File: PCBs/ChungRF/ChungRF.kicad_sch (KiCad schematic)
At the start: 11 parts, among them J1 Conn_Coaxial, J2 Conn_01x09_Socket, U1 E22-900M30S

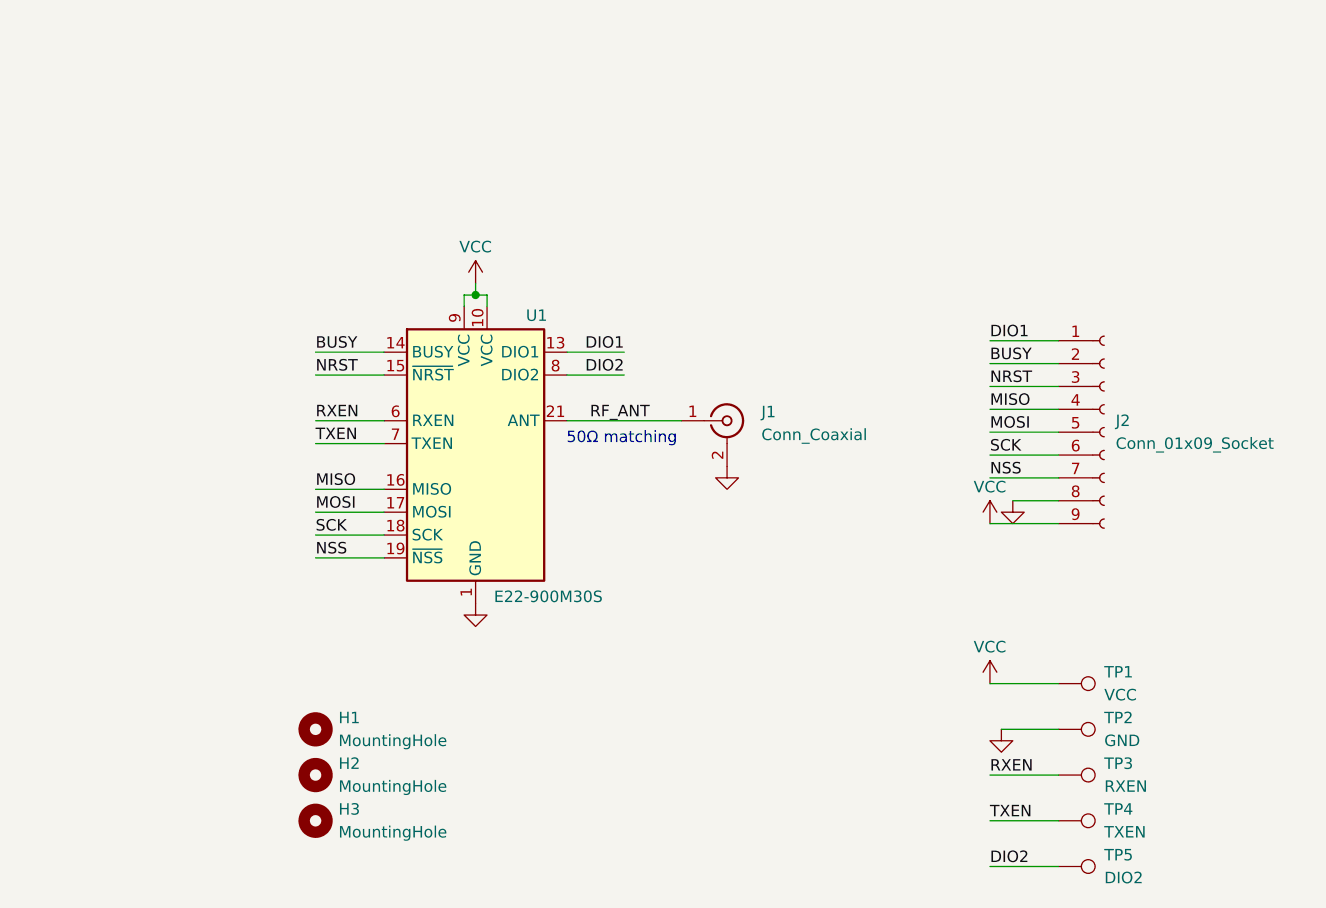
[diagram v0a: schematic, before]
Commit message: Rename to ChungRF
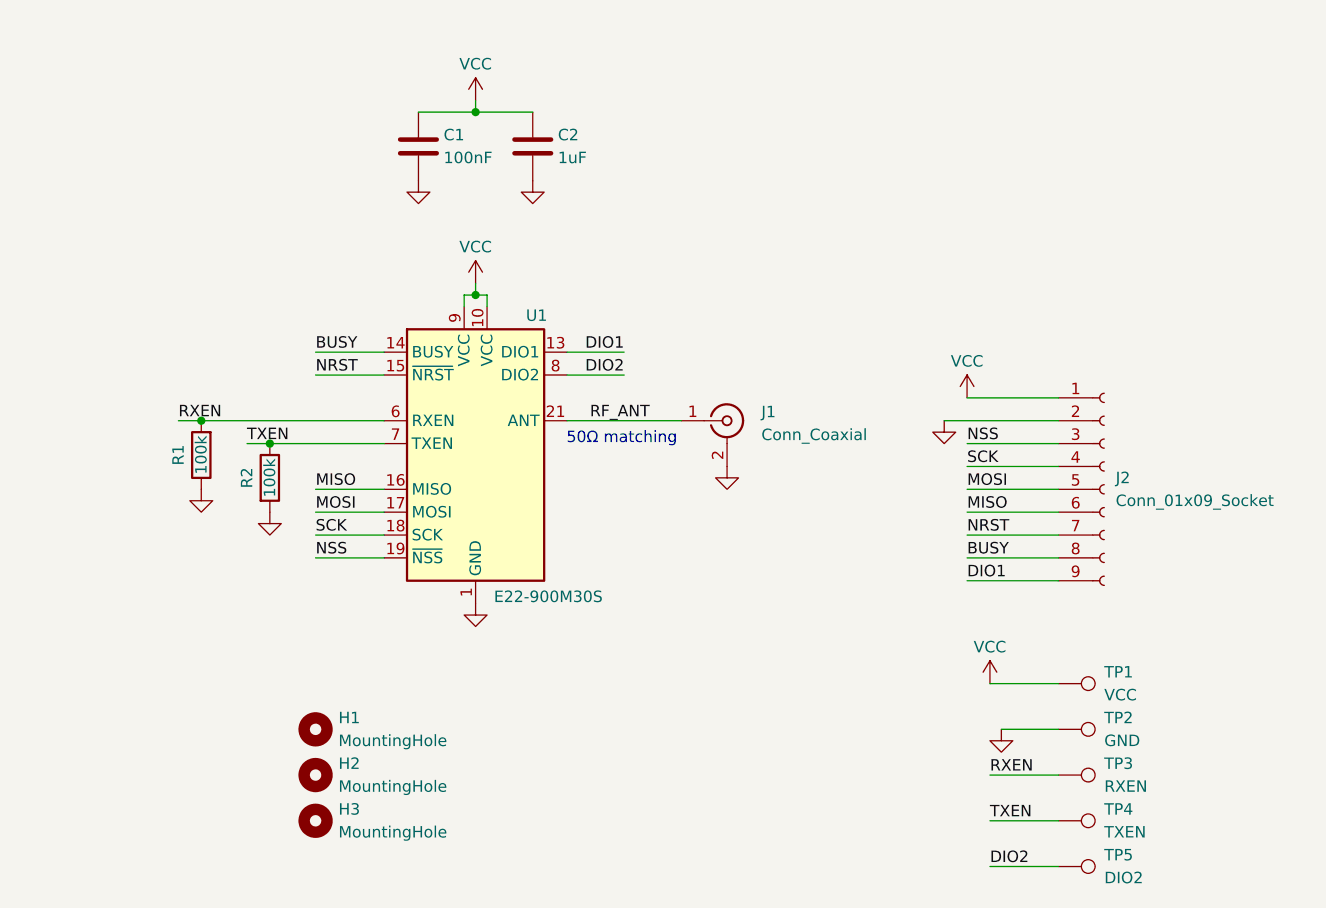
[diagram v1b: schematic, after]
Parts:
- added C1: 100nF, Capacitor_SMD:C_0603_1608Metric, symbol Device:C
- added C2: 1uF, Capacitor_SMD:C_0603_1608Metric, symbol Device:C
- added R1, R2: 100k, Capacitor_SMD:C_0603_1608Metric, symbol Device:R
- J2: footprint Connector_JST:JST_GH_BM09B-GHS-TBT_1x09-1MP_P1.25mm_Vertical -> Connector_JST:JST_SH_SM09B-SRSS-TB_1x09-1MP_P1.00mm_Horizontal
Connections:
- net BUSY: now also J2.8 (Pin_8); no longer J2.2 (Pin_2)
- net DIO1: now also J2.9 (Pin_9); no longer J2.1 (Pin_1)
- net GND: now also J2.2 (Pin_2), C1.2, C2.2, R1.1, R2.2; no longer J2.8 (Pin_8)
- net MISO: now also J2.6 (Pin_6); no longer J2.4 (Pin_4)
- net NRST: now also J2.7 (Pin_7); no longer J2.3 (Pin_3)
- net NSS: now also J2.3 (Pin_3); no longer J2.7 (Pin_7)
- net RXEN: now also R1.2
- net SCK: now also J2.4 (Pin_4); no longer J2.6 (Pin_6)
- net TXEN: now also R2.1
- net VCC: now also J2.1 (Pin_1), C1.1, C2.1; no longer J2.9 (Pin_9)
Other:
- moved on the sheet: J2

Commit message: Update ChungRF
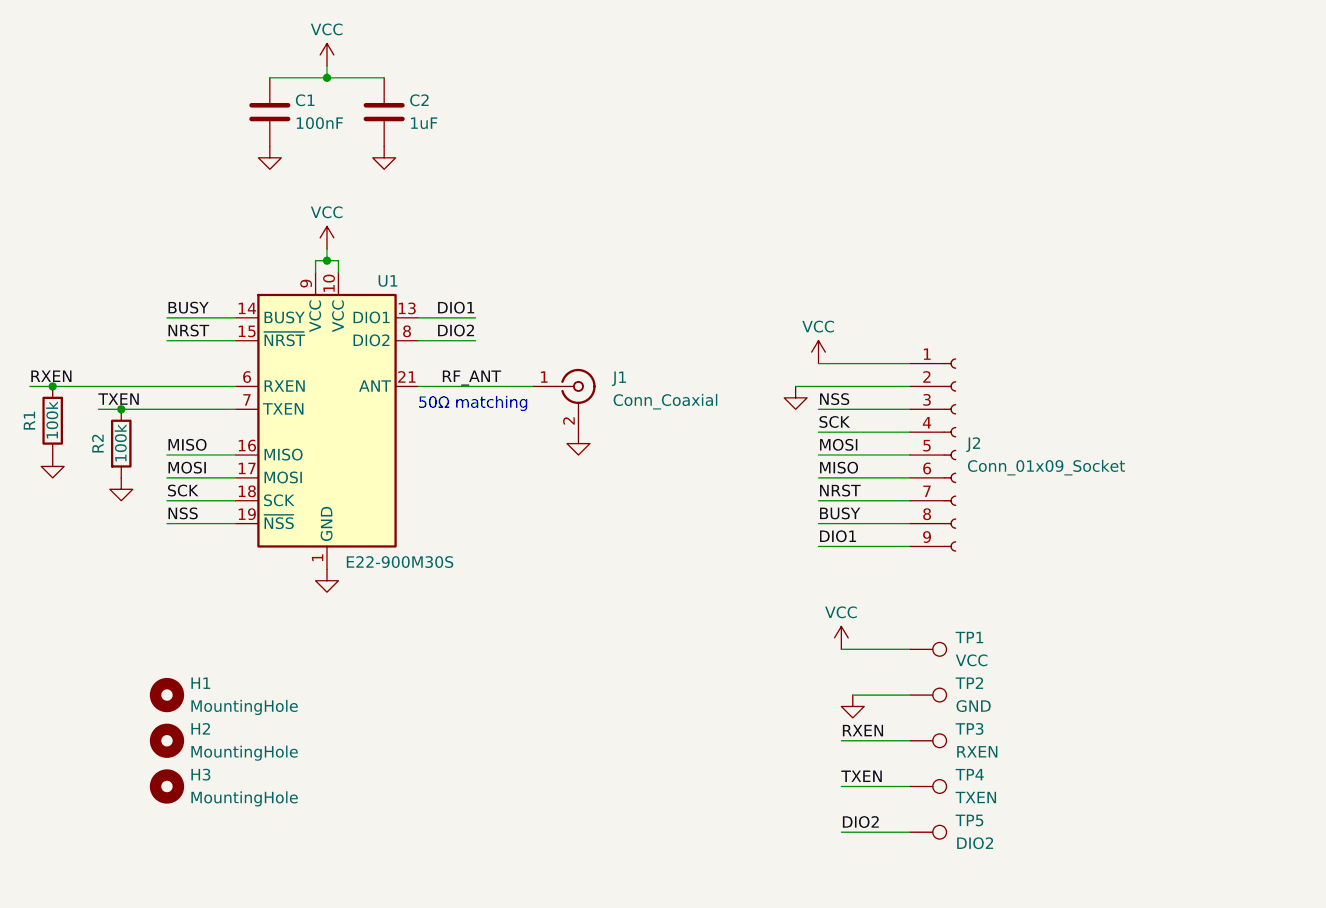
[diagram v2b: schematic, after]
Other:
- moved on the sheet: C1, C2, H1, H2, H3, J1, J2, R1, R2, TP1, TP2, TP3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
